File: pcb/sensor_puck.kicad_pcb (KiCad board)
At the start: 2 copper layers, 42.2 x 41.9 mm, 64 parts, among them J1 DISP LEFT, J2 DISP RIGHT, J3 USB_C_Receptacle_USB2.0_16P, J5 Generic, SW1 RST, SW2 BOOT, U1 ESP32-S3-MINI-1U, U2 LIS3MDL, U3 LSM6DSOXTR, U4 STC31-C-R3, U5 RT9013, U6 BME688

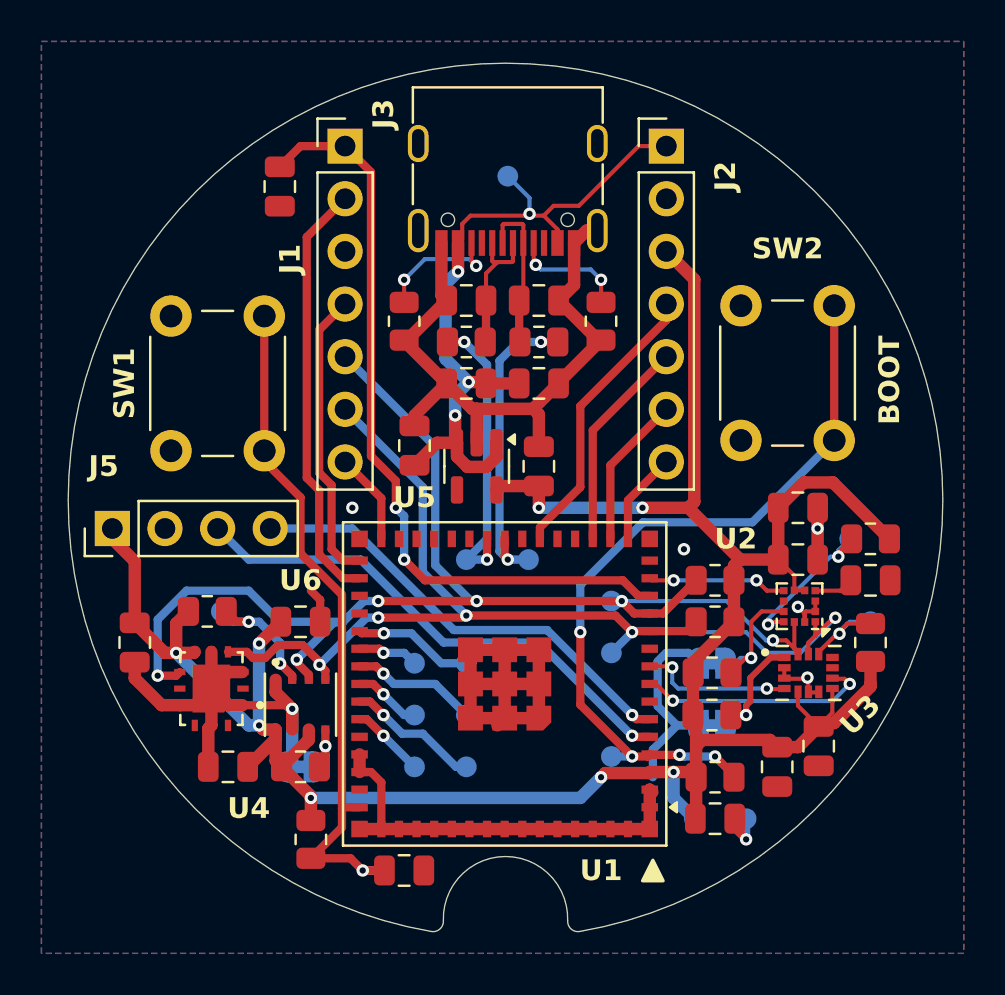
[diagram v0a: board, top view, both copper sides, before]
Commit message: feat: PCB design v0.2
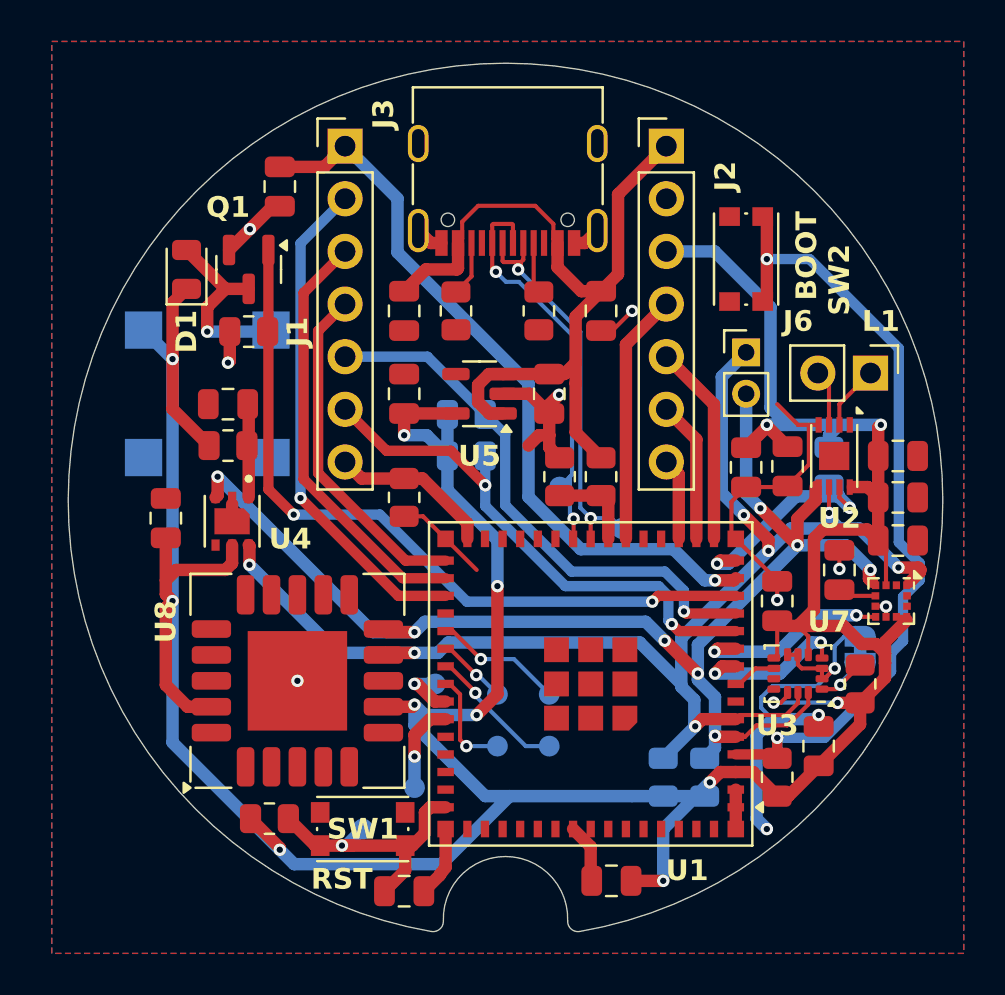
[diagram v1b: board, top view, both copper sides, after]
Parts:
- removed C11, C14, C15, C16: 100nF, Capacitor_SMD:C_0805_2012Metric
- removed J5: Generic, Connector_PinHeader_2.54mm:PinHeader_1x04_P2.54mm_Vertical
- removed JP1: LIS_SA1, Jumper:SolderJumper-2_P1.3mm_Bridged_RoundedPad1.0x1.5mm
- removed JP3: BME_SDO, Jumper:SolderJumper-2_P1.3mm_Bridged_RoundedPad1.0x1.5mm
- removed R13: 10k, Resistor_SMD:R_0805_2012Metric
- removed R14: 0R, Resistor_SMD:R_0805_2012Metric
- removed TP13: LIS_CS, TestPoint:TestPoint_Pad_D1.0mm
- removed TP14: LSM_CS, TestPoint:TestPoint_Pad_D1.0mm
- removed TP15: BME_CSB, TestPoint:TestPoint_Pad_D1.0mm
- removed TP3: 3V3, TestPoint:TestPoint_Pad_D1.0mm
- removed TP4: GND, TestPoint:TestPoint_Pad_D1.0mm
- removed TP7: SCL, TestPoint:TestPoint_Pad_D1.0mm
- removed TP8: SDA, TestPoint:TestPoint_Pad_D1.0mm
- removed TP9: VBUS, TestPoint:TestPoint_Pad_D1.0mm
- removed U6: BME688, BME688:IC_BME688
- added BZ1: Buzzer, Buzzer_Beeper:CMT-7525-80-SMT-TR, B.Cu at (85.5, 95.0)
- added C17: 220nF, Capacitor_SMD:C_0805_2012Metric, F.Cu at (116.0, 103.5)
- added C18: 100nF, Capacitor_SMD:C_0805_2012Metric, F.Cu at (118.8, 100.0)
- added C20: 100nF, Capacitor_SMD:C_0805_2012Metric, F.Cu at (118.8, 102.1)
- added C21: 10nF, Capacitor_SMD:C_0805_2012Metric, F.Cu at (118.8, 98.0)
- added D1: D, Diode_SMD:D_0805_2012Metric, F.Cu at (84.5, 89.0)
- added J6: Conn_01x02_Socket, Connector_PinHeader_2.00mm:PinHeader_1x02_P2.00mm_Vertical, F.Cu at (111.5, 93.0)
- added L1: TBD, Connector_PinHeader_2.54mm:PinHeader_1x02_P2.54mm_Vertical, F.Cu at (117.5, 94.0)
- added Q1: 2N7002, Package_TO_SOT_SMD:SOT-23, F.Cu at (87.5, 89.0)
- added R15: 10k, Resistor_SMD:R_0805_2012Metric, F.Cu at (102.5, 99.0)
- added R16: 10k, Resistor_SMD:R_0805_2012Metric, B.Cu at (98.0, 96.0)
- added R17: 10k, Resistor_SMD:R_0805_2012Metric, B.Cu at (98.0, 98.0)
- added U7: LIS2MDL, Package_LGA:LGA-12_2x2mm_P0.5mm, F.Cu at (118.5, 105.0)
- added U8: SCD41-D-R2, Sensor:Sensirion_SCD4x-1EP_10.1x10.1mm_P1.25mm_EP4.8x4.8mm, F.Cu at (89.8, 108.8)
- C10: value 1uF -> 10nF
- C4, C5: value DNP -> 1uF
- R10: value 0R -> 10k
- R11: value 0R -> 5k11
- R2, R3: moved to B.Cu
- R8: value 0 -> 10k; moved to B.Cu
- R9: value 0 -> 4R7
- SW1, SW2: footprint Button_Switch_THT:SW_PUSH_6mm -> Button_Switch_SMD:SW_Push_1P1T_NO_CK_KMR2
- U2: value LIS3MDL -> ST25DV16K-IER8C3; footprint Package_LGA:LGA-12_2x2mm_P0.5mm -> Package_DFN_QFN:DFN-8-1EP_3x2mm_P0.5mm_EP1.36x1.46mm
- U3: footprint LSM6DSOX:PQFN50P250X300X86-14N -> Package_LGA:LGA-14_3x2.5mm_P0.5mm_LayoutBorder3x4y
- U4: value STC31-C-R3 -> SGP41-D-R4; footprint STC31-C:XDCR_STC31-C-R3 -> SGP41-D-R4:XDCR_SGP41-D-R4
- moved R4 27.8 mm to (87.5, 92.0)
- moved R10 22.6 mm to (95.0, 100.0), turned to -90 degrees
- moved C5 20.8 mm to (83.5, 101.0), turned to 90 degrees
- moved SW1 20.5 mm to (93.0, 116.0), turned to 0 degrees
- moved R11 15.3 mm to (104.5, 99.0), turned to -90 degrees
- moved R8 15.2 mm to (115.5, 98.5), turned to 90 degrees
- moved C4 12.5 mm to (86.5, 95.5)
- moved R9 12.5 mm to (86.5, 97.5), turned to 180 degrees
- moved R3 9.82 mm to (107.5, 113.5), turned to -90 degrees
- moved SW2 8.75 mm to (111.5, 88.5), turned to -90 degrees
- moved U4 8.14 mm to (86.7, 101.2), turned to -90 degrees
- moved JP2 8.03 mm to (117.0, 107.3), turned to 90 degrees
- moved C13 8.00 mm to (113.0, 105.0), turned to -90 degrees
- moved TP6 8.00 mm to (113.0, 112.5)
- moved R2 7.52 mm to (109.5, 113.5), turned to 90 degrees
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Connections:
- C4 pad 1: Net-(C4-Pad1) -> Net-(U4-VDD)
- C5 pad 1: Net-(C5-Pad1) -> +3V3
- C9 pad 1: Net-(U2-C1) -> GND
- C9 pad 2: GND -> +3V3
- J1 pad 3: unconnected-(J1-Pin_3-Pad3) -> SD_CS
- J1 pad 5: I2C_SDA -> LCD_I2C_SDA
- J1 pad 6: I2C_SCL -> LCD_I2C_SCL
- J3 pad A6: Net-(C4-Pad1) -> USB_D+
- J3 pad A7: Net-(C5-Pad1) -> USB_D-
- J3 pad B6: Net-(C4-Pad1) -> USB_D+
- J3 pad B7: Net-(C5-Pad1) -> USB_D-
- R10 pad 1: +3V3 -> LCD_BL
- R10 pad 2: Net-(U2-~{CS}) -> GND
- R11 pad 1: +3V3 -> VBUS
- R11 pad 2: Net-(U3-CS) -> Net-(U1-IO18)
- R2 pad 1: I2C_SCL -> +3V3
- R2 pad 2: +3V3 -> I2C_SDA
- R3 pad 1: +3V3 -> I2C_SCL
- R3 pad 2: I2C_SDA -> +3V3
- R4 pad 1: Net-(JP1-B) -> BUZZER_EN
- R4 pad 2: +3V3 -> GND
- R8 pad 1: Net-(C5-Pad1) -> ST25DV_INT
- R8 pad 2: USB_D- -> +3V3
- R9 pad 1: USB_D+ -> Net-(U4-VDD)
- R9 pad 2: Net-(C4-Pad1) -> +3V3
- SW2 pad 1: GND -> IO0
- SW2 pad 2: IO0 -> GND
- U1 pad 10: unconnected-(U1-IO6-Pad10) -> LIS2_INT
- U1 pad 11: I2C_SCL -> LCD_I2C_SCL
- U1 pad 12: I2C_SDA -> LCD_I2C_SDA
- U1 pad 13: BATT_READ -> BUZZER_EN
- U1 pad 14: LIS3_INT -> BATT_READ
- U1 pad 15: unconnected-(U1-IO11-Pad15) -> ST25DV_INT
- U1 pad 16: TP_INT -> MISO
- U1 pad 18: MISO -> TP_INT
- U1 pad 22: unconnected-(U1-IO18-Pad22) -> Net-(U1-IO18)
- U1 pad 32: LCD_CS -> SD_CS
- U1 pad 33: unconnected-(U1-IO37-Pad33) -> LCD_CS
- U1 pad 5: IO1 -> I2C_SDA
- U1 pad 6: IO2 -> I2C_SCL
- U2 pad 1: I2C_SCL -> unconnected-(U2-V_EH-Pad1)
- U2 pad 2: GND -> Net-(U2-AC0)
- U2 pad 3: GND -> Net-(U2-AC1)
- U2 pad 4: Net-(U2-C1) -> GND
- U2 pad 5: +3V3 -> I2C_SDA
- U2 pad 6: +3V3 -> I2C_SCL
- U2 pad 7: LIS3_INT -> ST25DV_INT
- U2 pad 8: unconnected-(U2-DRDY-Pad8) -> +3V3
- U2 pad 9: Net-(JP1-B) -> unconnected-(U2-NC-Pad9)
- U3 pad 12: Net-(U3-CS) -> +3V3
- U4 pad 1: GND -> Net-(U4-VDD)
- U4 pad 2: unconnected-(U4-RESERVED-Pad2) -> GND
- U4 pad 3: GND -> I2C_SDA
- U4 pad 4: I2C_SCL -> GND
- U4 pad 5: GND -> +3V3
- U4 pad 6: +3V3 -> I2C_SCL
- U4 pad 7: I2C_SDA -> GND
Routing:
- net +3V3: track 122.8 -> 187.7 mm, vias 8 -> 13
- net GND: track 116.0 -> 66.9 mm, vias 7 -> 11
- net BUZZER_EN: track 0.00 -> 36.5 mm, vias 0 -> 2
- net LCD_I2C_SDA: track 0.00 -> 26.6 mm, vias 0 -> 1
- net LCD_I2C_SCL: track 0.00 -> 26.0 mm, vias 0 -> 2
- net IO1: track 25.0 -> 0.00 mm, vias 1 -> 0
- net IO2: track 22.1 -> 0.00 mm, vias 1 -> 0
- net SD_CS: track 0.00 -> 20.6 mm
- net Net-(U1-EN): track 33.7 -> 13.9 mm
- net I2C_SCL: track 53.6 -> 67.3 mm, vias 5 -> 7
- net ST25DV_INT: track 0.00 -> 11.1 mm, vias 0 -> 2
- net LIS2_INT: track 0.00 -> 9.83 mm, vias 0 -> 2
- net Net-(BZ1--): track 0.00 -> 9.31 mm, vias 0 -> 1
- net LSM6_INT2: track 11.3 -> 2.15 mm, vias 2 -> 0
- net Net-(U2-~{CS}): track 7.92 -> 0.00 mm, vias 2 -> 0
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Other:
- board text added: "RST"
- board text added: "Sensor Puck v0.2"
- board text removed: "3V3"
- board text removed: "BME CSB"
- board text removed: "BME SDO"
- board text removed: "GND"
- board text removed: "LIS CS"
- board text removed: "LIS SA1"
- board text removed: "LSM CS"
- board text removed: "SCL"
- board text removed: "SDA"
